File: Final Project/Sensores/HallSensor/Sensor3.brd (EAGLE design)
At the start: 14.4 x 12.6 mm, 5 parts

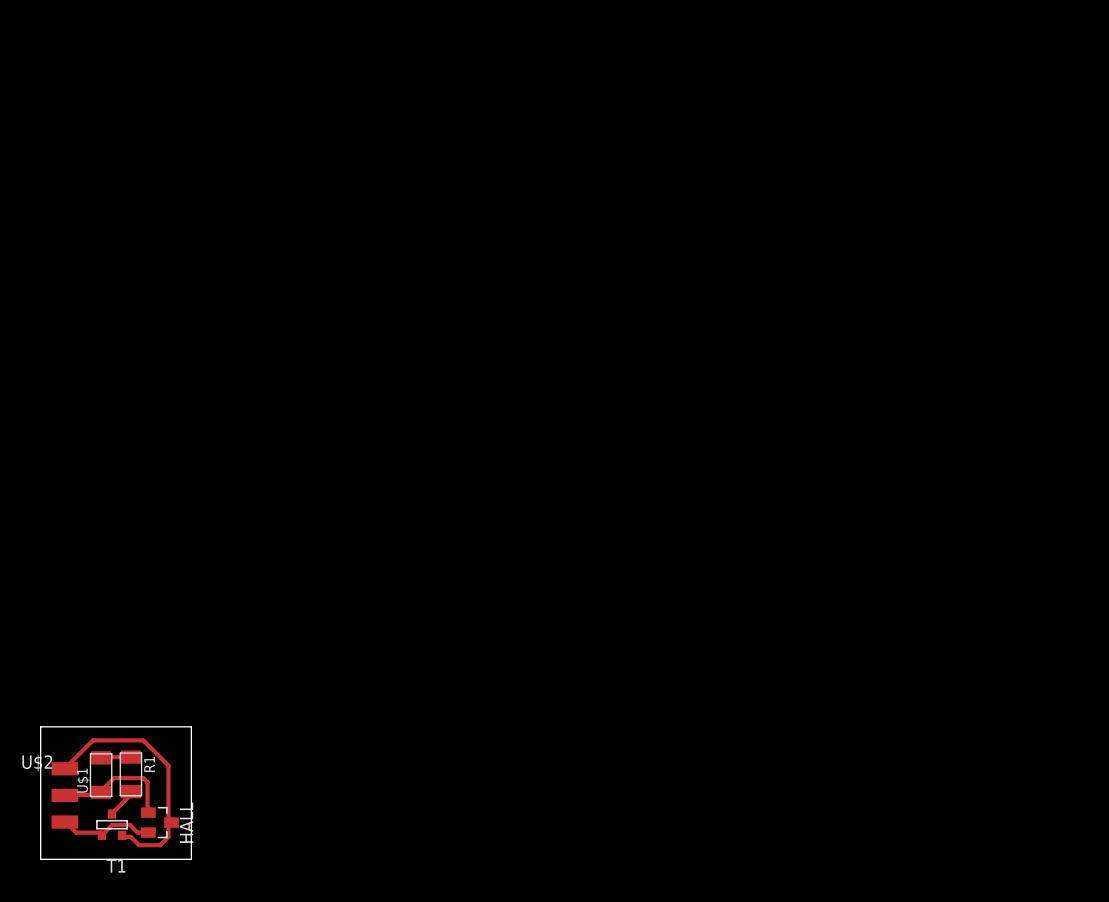
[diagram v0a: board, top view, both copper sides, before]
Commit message: sensor
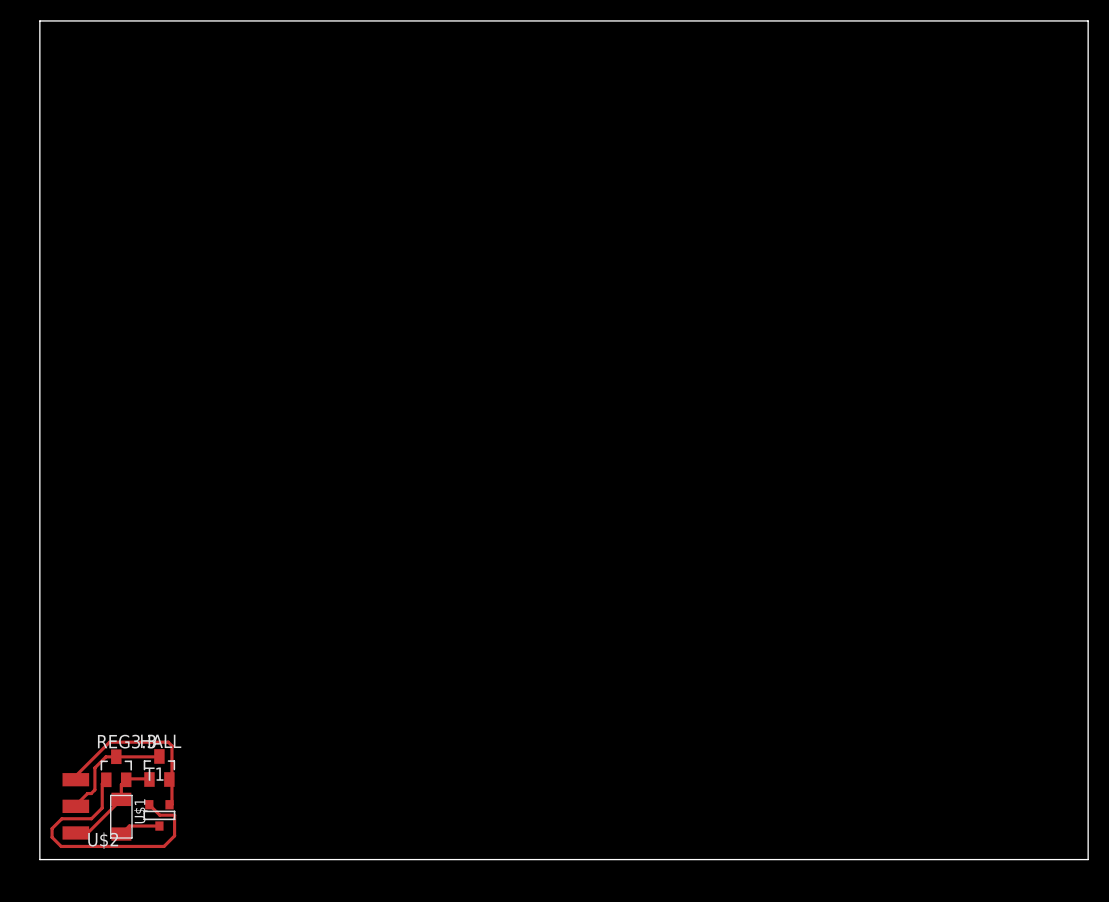
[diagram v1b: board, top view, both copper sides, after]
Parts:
- removed R1: (no value), fab:R1206FAB
- added REG3.3: (no value), fab:SOT23
- moved HALL 5.21 mm to (11.4, 8.74), turned to 0 degrees
- moved T1 4.56 mm to (11.4, 4.22), turned to 0 degrees
- moved U$1 4.41 mm to (7.77, 4.09), turned to 270 degrees
- moved U$2 2.08 mm to (3.81, 5.08), turned to 180 degrees
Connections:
- removed net N$1: R1.1, U$1.2
- removed net N$2: R1.2, T1.1
- new net 3.3V: REG3.3.1, T1.2
- new net IN: T1.1, U$1.2
- net GND: now also REG3.3.3, U$2.2; no longer T1.2, U$2.1
- net VCC: now also REG3.3.2, U$2.1; no longer U$2.2
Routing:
- net 3.3V: track 0.00 -> 26.6 mm
- net GND: track 24.3 -> 11.2 mm
- net ANALOG: track 9.30 -> 17.4 mm
- net IN: track 0.00 -> 3.95 mm
- net N$1: track 2.89 -> 0.00 mm
- net N$2: track 2.86 -> 0.00 mm
- net VCC: track 11.7 -> 9.98 mm
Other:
- board size 14.4 x 12.6 mm -> 100 x 80 mm
